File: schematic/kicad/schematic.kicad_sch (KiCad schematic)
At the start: 16 parts, among them J1 Conn_01x02_Pin, J2 Conn_01x02_Pin, Q1 AO3401, SW1 SW_Nidec_CAS-120A1, U1 ESP32-C3, U2 MAX4466, U3 HW-373, U4 MT3608, U5 WS2812B

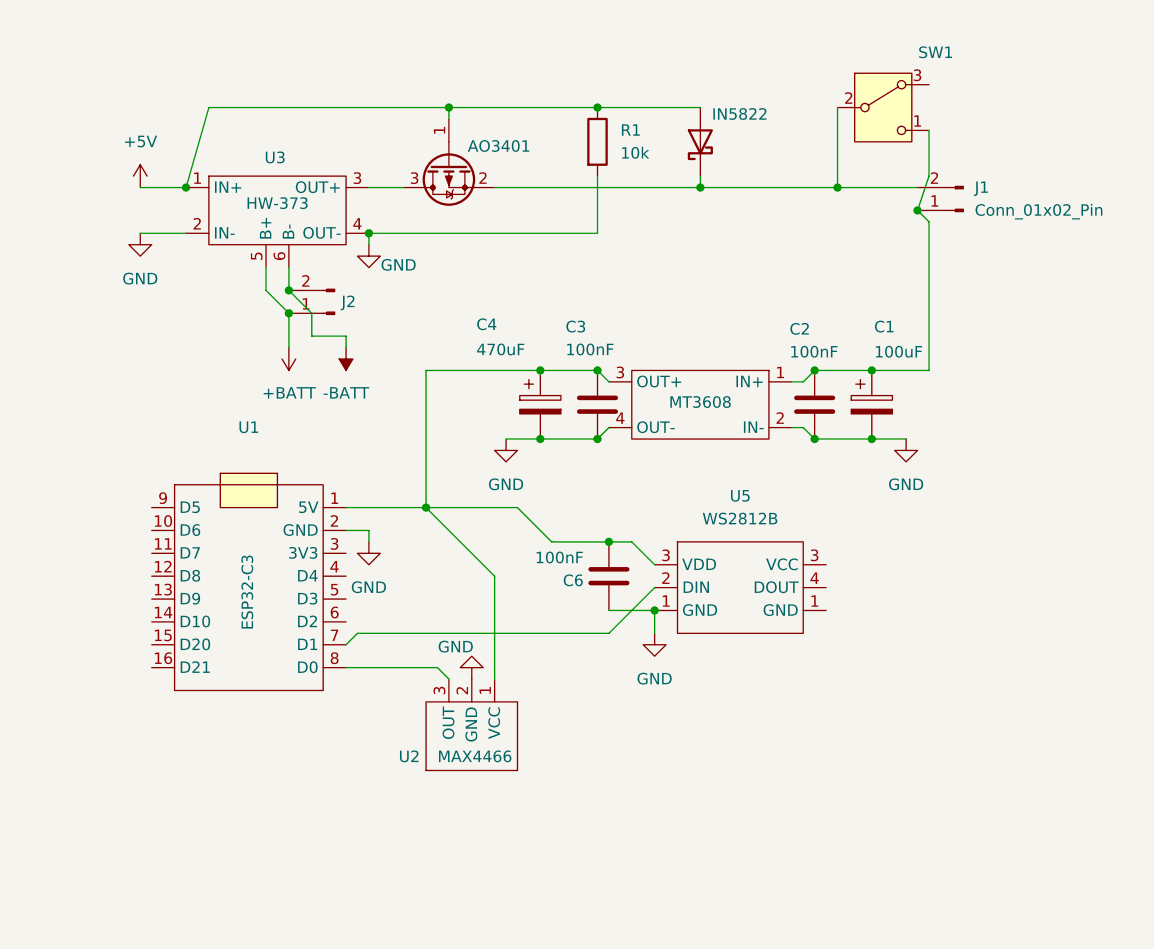
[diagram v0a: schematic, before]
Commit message: Adjust pcb and schematic
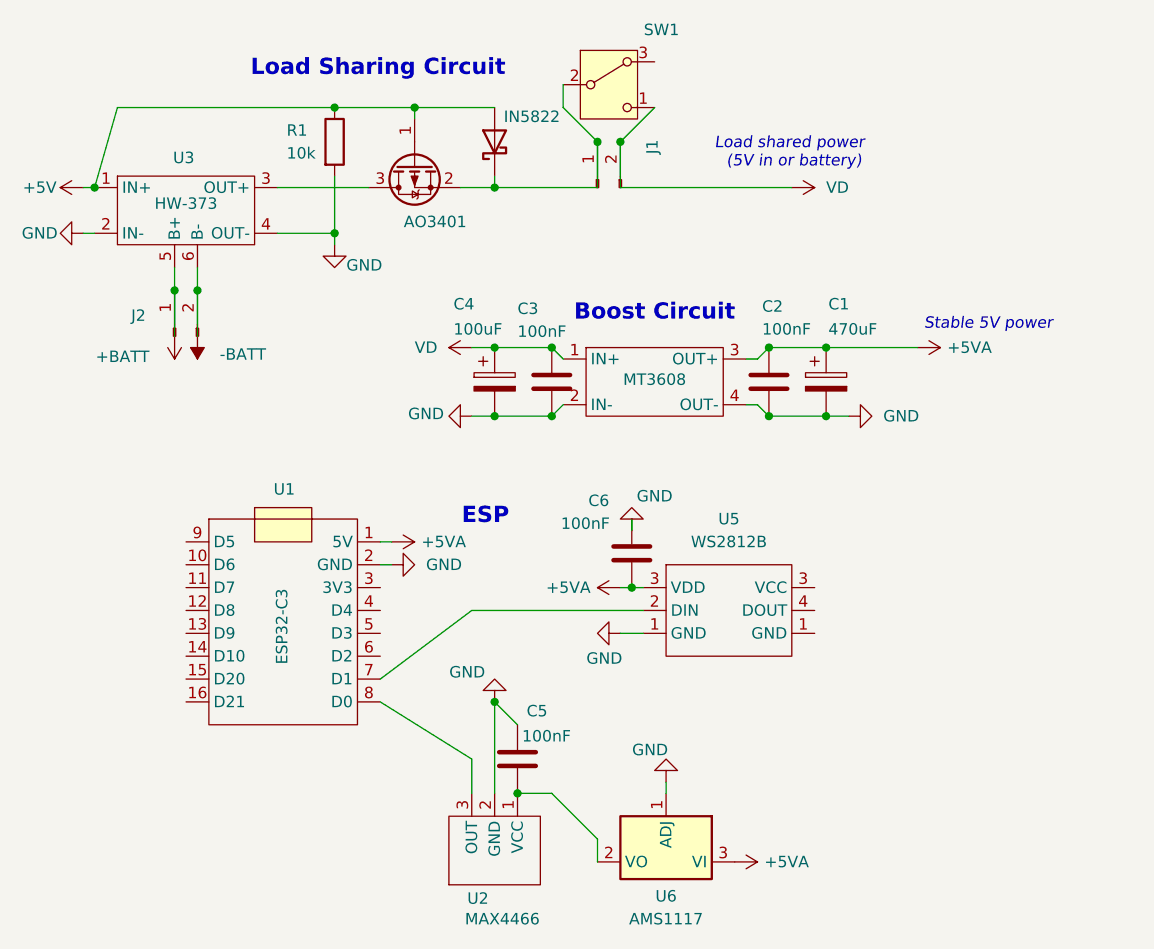
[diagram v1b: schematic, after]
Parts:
- added C5: 100nF, Capacitor_THT:C_Disc_D5.0mm_W2.5mm_P5.00mm, symbol Device:C
- added U6: AMS1117, Connector_PinHeader_2.54mm:PinHeader_1x03_P2.54mm_Vertical, symbol Regulator_Linear:AMS1117
- C1: value 100uF -> 470uF
- C4: value 470uF -> 100uF
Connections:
- net GND: now also C5.2, U6.1 (ADJ)
- net +5VA: now reaches C6.1, U1.1 (5V), U4.3 (OUT+), U5.3 (VCC)
- net +5VA: now also C1.1, C2.1, U6.3 (VI); no longer C3.1, C4.1, U2.1 (VCC)
- net at IN5822.1 (K), Q1.2 (S), SW1.2 (B): now also J1.1 (Pin_1); no longer J1.2 (Pin_2)
- new net: C5.1, U2.1 (VCC), U6.2 (VO)
- new net VD: C3.1, C4.1, J1.2 (Pin_2), SW1.1 (C), U4.1 (IN+)
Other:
- note added: "(5V in or battery)"
- note added: "Boost Circuit"
- note added: "ESP"
- note added: "Load Sharing Circuit"
- note added: "Load shared power"
- note added: "Stable 5V power"
- moved on the sheet: C1, C2, C3, C4, C6, IN5822, J1, J2, R1, SW1, U1, U2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
